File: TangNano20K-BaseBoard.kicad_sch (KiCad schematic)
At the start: 49 parts, among them J1 Conn_01x20_Socket, J2 Conn_01x20_Socket, J3 Conn_01x06_Socket, J4 Conn_01x06_Socket, Q1 PN2222A, Q2 PN2222A, Q3 PN2222A, Q4 PN2222A, U1 CC56-12EWA, U2 SSD1306

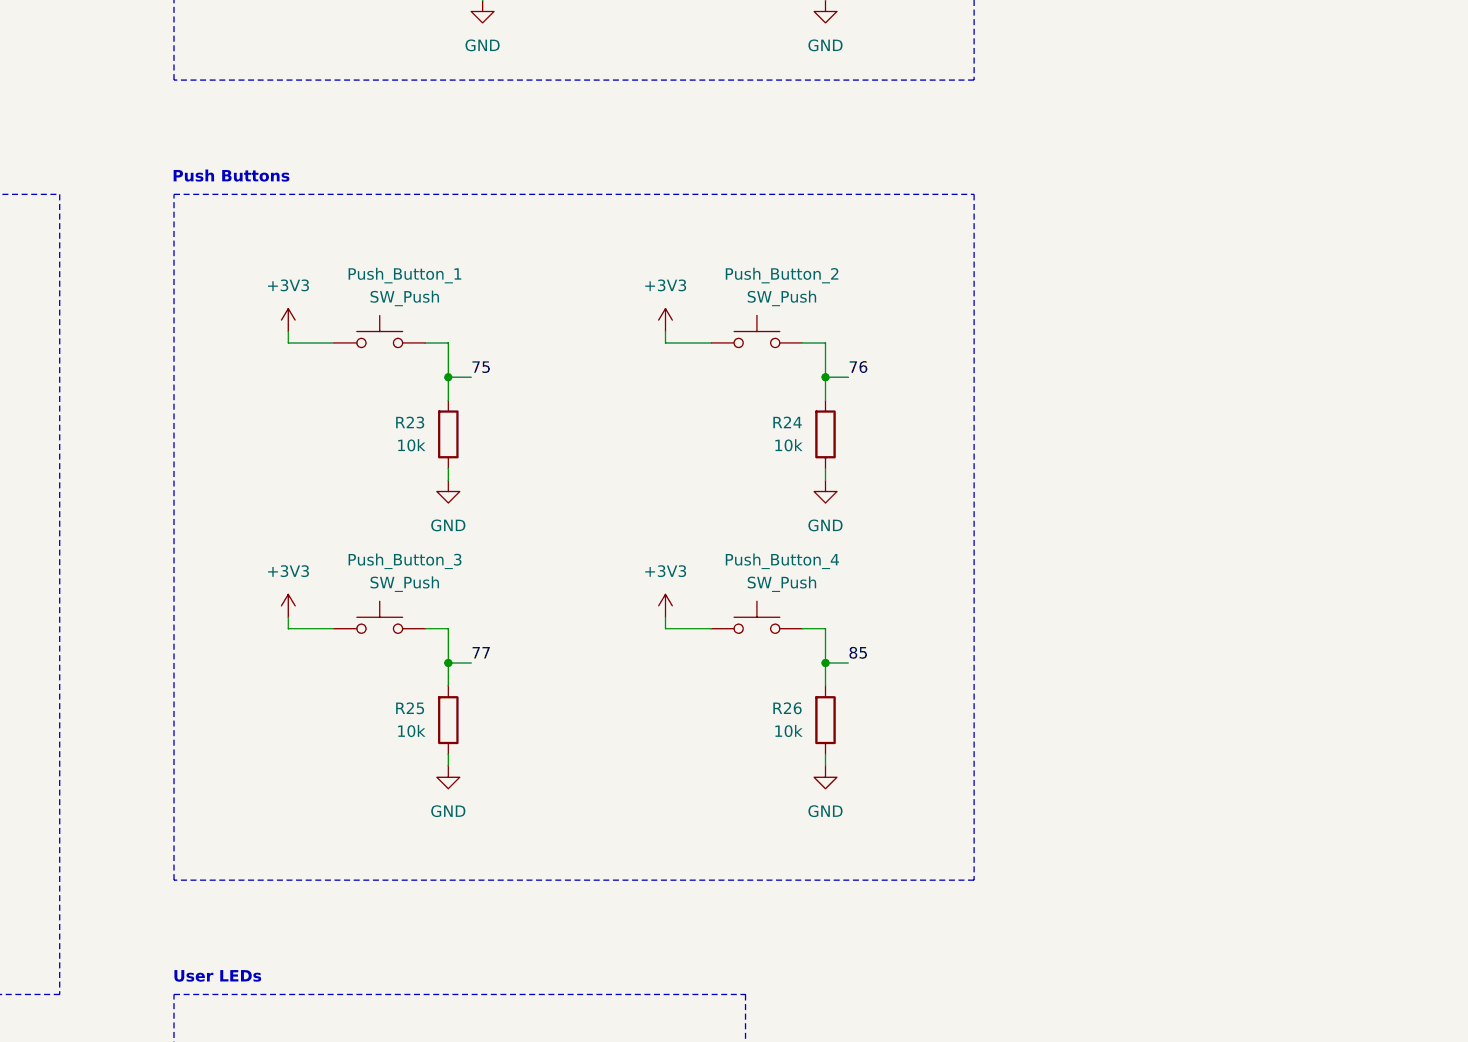
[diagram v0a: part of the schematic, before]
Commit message: Update schematic, add new symbol, footprint and 3d model
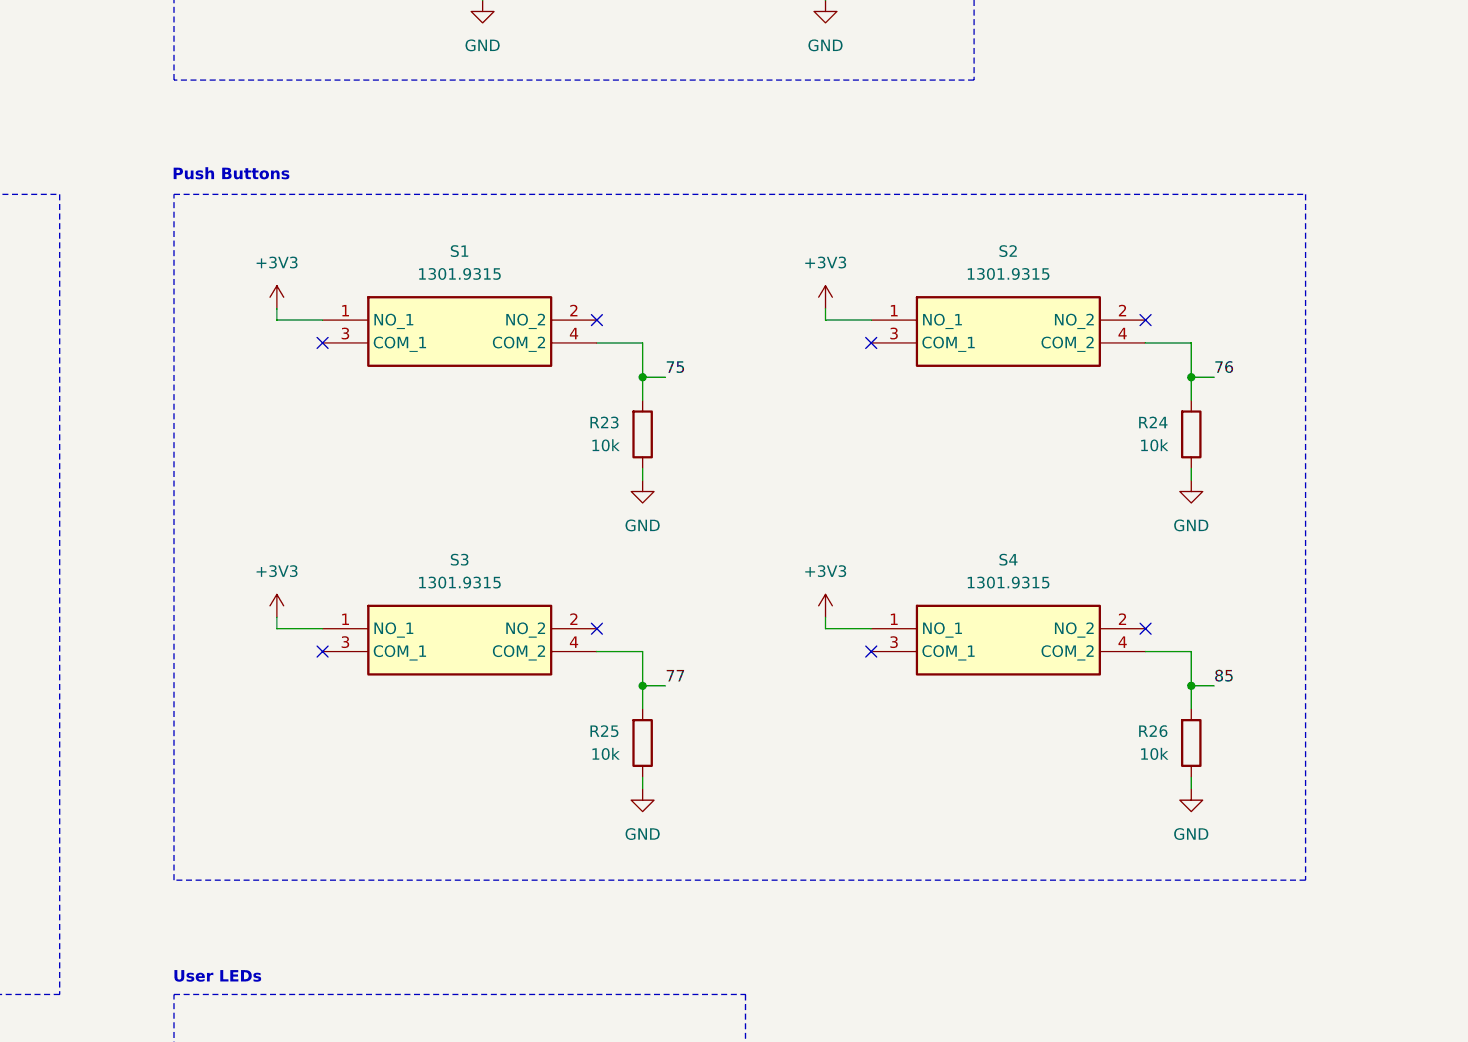
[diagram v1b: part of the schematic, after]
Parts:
- removed Push_Button_1, Push_Button_2, Push_Button_3, Push_Button_4: SW_Push, Button_Switch_SMD:SW_Push_1TS009xxxx-xxxx-xxxx_6x6x5mm, symbol Switch:SW_Push
- added S1, S2, S3, S4: 1301.9315, MyFootPrints:13019319, symbol MySymbols:1301.9315
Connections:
- net +3V3: now also S1.1 (NO_1), S2.1 (NO_1), S3.1 (NO_1), S4.1 (NO_1)
- net 75: now also S1.4 (COM_2)
- net 76: now also S2.4 (COM_2)
- net 77: now also S3.4 (COM_2)
- net 85: now also S4.4 (COM_2)
- no-connect marks 5 -> 13
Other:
- moved on the sheet: R23
